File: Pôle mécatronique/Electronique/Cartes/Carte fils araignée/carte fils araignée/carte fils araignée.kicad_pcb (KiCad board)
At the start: 2 copper layers, 27 x 79 mm, 22 parts, among them J1 Conn_01x05, J10 Conn_01x05, J11 Conn_01x05, J12 Conn_01x05, J13 Conn_01x05, J2 Conn_01x05, J3 Conn_01x05, J4 Conn_01x05, J5 X3, J6 X1, J7 Conn_01x05, J8 X2, J9 Conn_01x04

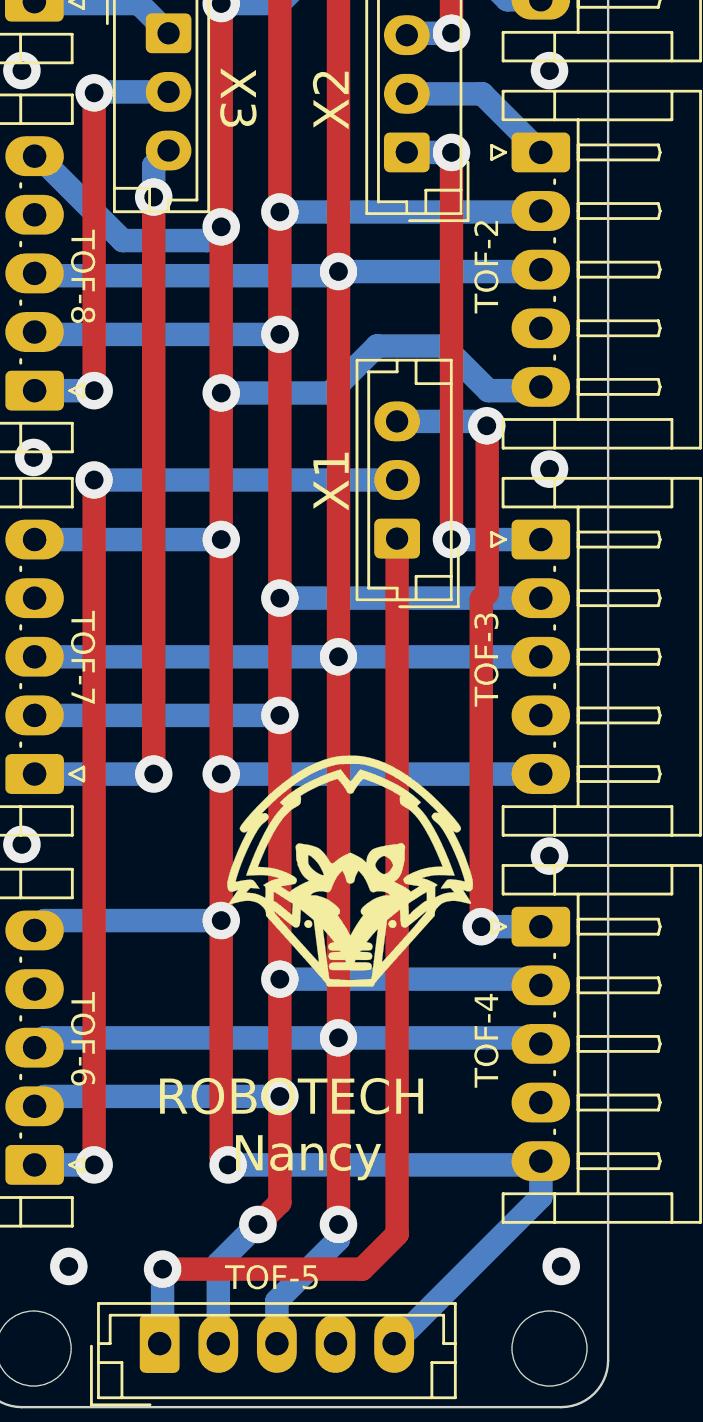
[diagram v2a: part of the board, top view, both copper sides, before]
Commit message: Version finale JLCPCB
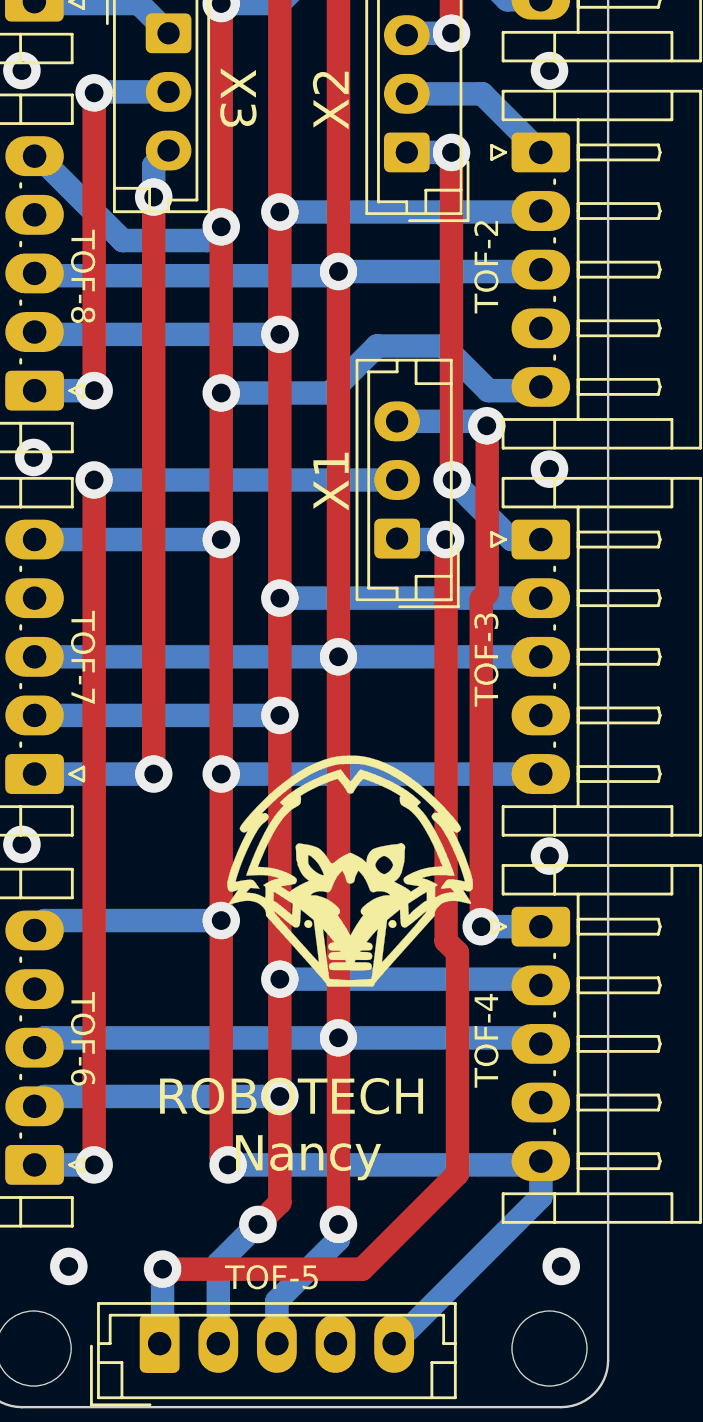
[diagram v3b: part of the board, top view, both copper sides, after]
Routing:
- net Xshut5: track 43.5 -> 46.8 mm, vias 1 -> 2
- net Xshut3: track 22.2 -> 20.7 mm
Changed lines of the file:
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@@
   (segment (start 145 124.46) (end 132.08 124.46) (width 1) (layer "B.Cu") (net 8))
   (segment (start 132.08 153.67) (end 129.54 153.67) (width 1) (layer "B.Cu") (net 8))
-  (segment (start 143.51 158.115) (end 145 156.625) (width 1) (layer "F.Cu") (net 9))
-  (segment (start 145 156.625) (end 145 126.96) (width 1) (layer "F.Cu") (net 9))
-  (segment (start 135 158.115) (end 143.51 158.115) (width 1) (layer "F.Cu") (net 9))
+  (segment (start 147.090489 127.024489) (end 147.090489 144.131119) (width 1) (layer "F.Cu") (net 9))
+  (segment (start 143.51 158.115) (end 135 158.115) (width 1) (layer "F.Cu") (net 9))
+  (segment (start 147.574 144.61463) (end 147.574 154.051) (width 1) (layer "F.Cu") (net 9))
+  (segment (start 147.090489 144.131119) (end 147.574 144.61463) (width 1) (layer "F.Cu") (net 9))
+  (segment (start 147.066 127) (end 147.090489 127.024489) (width 1) (layer "F.Cu") (net 9))
+  (segment (start 147.574 154.051) (end 143.51 158.115) (width 1) (layer "F.Cu") (net 9))
+  (via (at 147.066 127) (size 1.6) (drill 0.8) (layers "F.Cu" "B.Cu") (net 9))
   (via (at 135 158.115) (size 1.6) (drill 0.8) (layers "F.Cu" "B.Cu") (net 9))
   (segment (start 135 158.115) (end 135 161.164) (width 1) (layer "B.Cu") (net 9))
   (segment (start 135 161.164) (end 134.874 161.29) (width 1) (layer "B.Cu") (net 9))
+  (segment (start 145.04 127) (end 145 126.96) (width 1) (layer "B.Cu") (net 9))
+  (segment (start 147.066 127) (end 145.04 127) (width 1) (layer "B.Cu") (net 9))
   (segment (start 148.824951 122.147972) (end 148.844 122.167021) (width 1) (layer "F.Cu") (net 10))
   (segment (start 148.59 129.54) (end 148.59 143.51) (width 1) (layer "F.Cu") (net 10))
@@
   (segment (start 148.59 143.51) (end 151.13 143.51) (width 1) (layer "B.Cu") (net 10))
   (segment (start 148.636979 121.96) (end 145 121.96) (width 1) (layer "B.Cu") (net 10))
-  (segment (start 147.32 127) (end 147.32 110.49) (width 1) (layer "F.Cu") (net 11))
+  (segment (start 147.3445 124.46) (end 147.32 124.4355) (width 1) (layer "F.Cu") (net 11))
+  (segment (start 147.32 124.4355) (end 147.32 110.49) (width 1) (layer "F.Cu") (net 11))
   (via (at 147.32 110.49) (size 1.6) (drill 0.8) (layers "F.Cu" "B.Cu") (net 11))
-  (via (at 147.32 127) (size 1.6) (drill 0.8) (layers "F.Cu" "B.Cu") (net 11))
-  (segment (start 151.13 127) (end 147.32 127) (width 1) (layer "B.Cu") (net 11))
+  (via (at 147.3445 124.46) (size 1.6) (drill 0.8) (layers "F.Cu" "B.Cu") (net 11))
+  (segment (start 149.8845 127) (end 147.3445 124.46) (width 1) (layer "B.Cu") (net 11))
   (segment (start 147.32 110.49) (end 145.415 110.49) (width 1) (layer "B.Cu") (net 11))
+  (segment (start 151.13 127) (end 149.8845 127) (width 1) (layer "B.Cu") (net 11))
   (segment (start 145.415 107.99) (end 148.63 107.99) (width 1) (layer "B.Cu") (net 12))
   (segment (start 148.63 107.99) (end 151.13 110.49) (width 1) (layer "B.Cu") (net 12))
